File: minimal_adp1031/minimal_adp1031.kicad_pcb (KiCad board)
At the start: 4 copper layers, 39.6 x 27.9 mm, 34 parts, among them T1 ZA9644-AED, U1 ADP1031ACPZ-3-R7

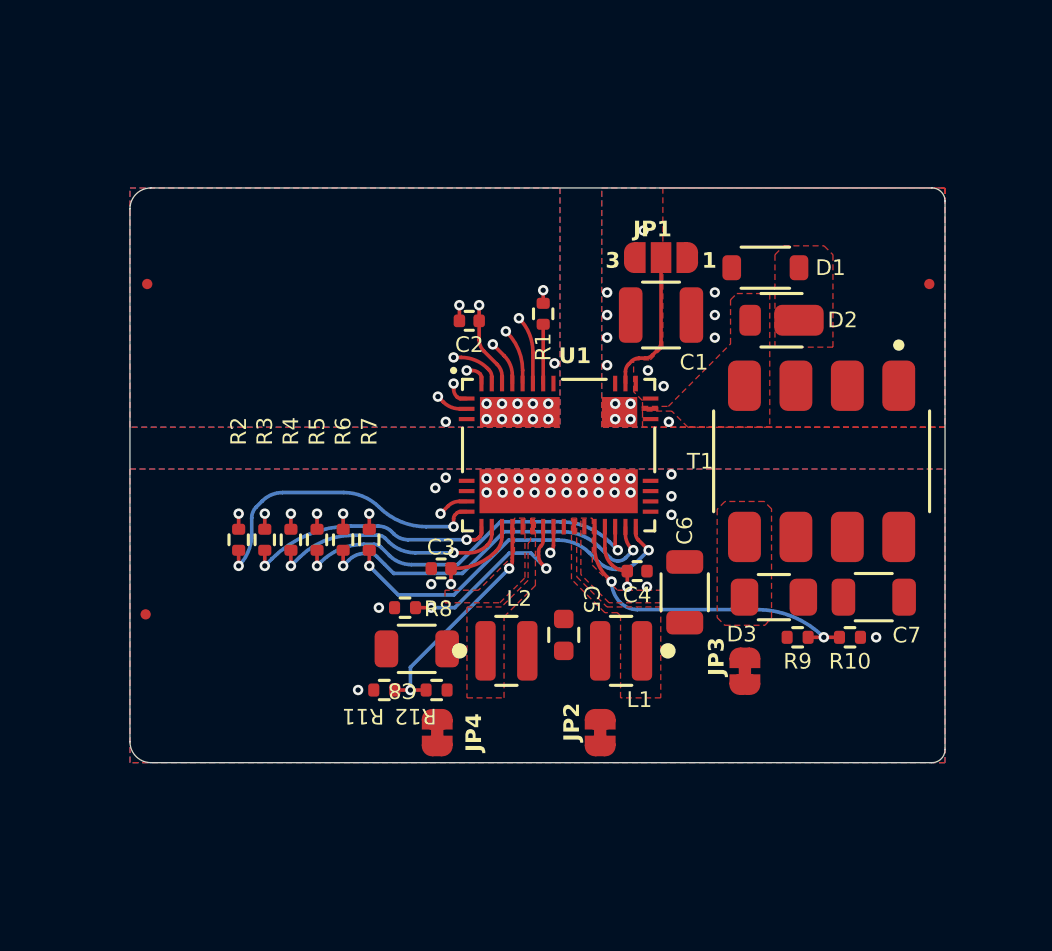
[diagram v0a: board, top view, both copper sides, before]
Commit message: backup
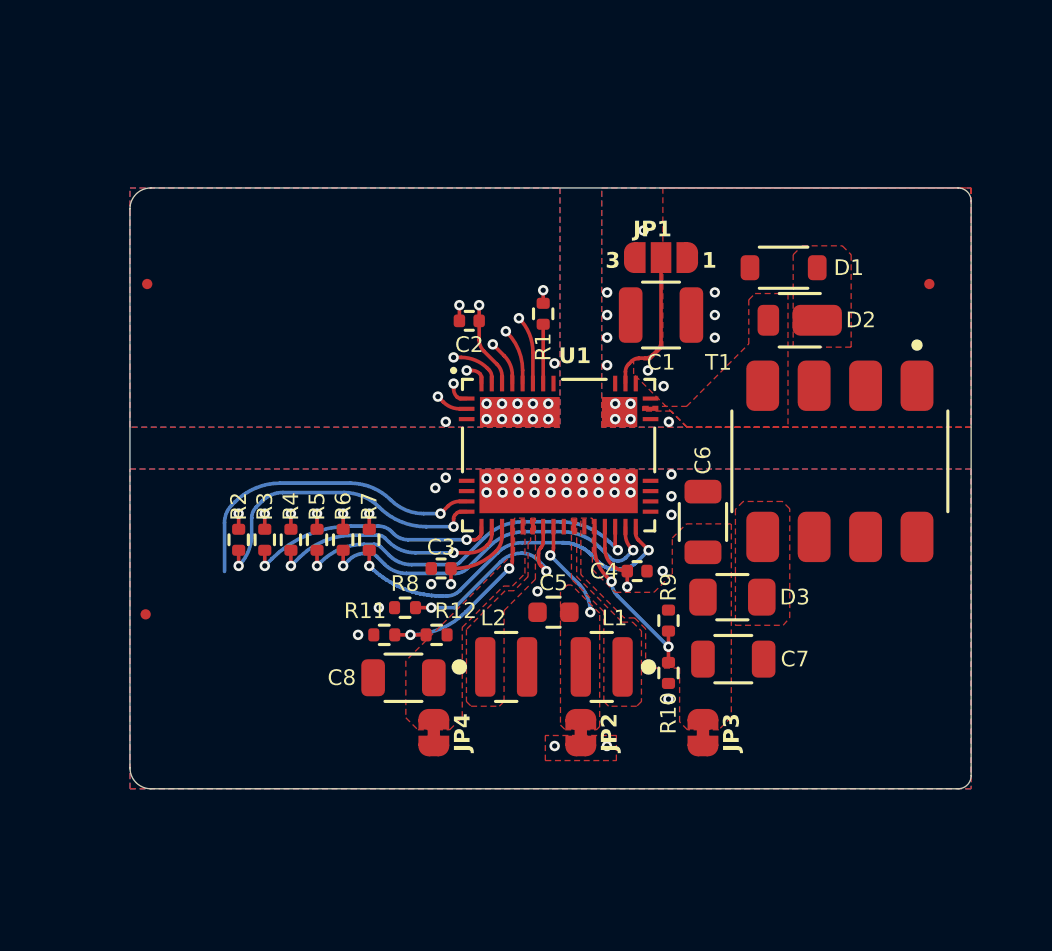
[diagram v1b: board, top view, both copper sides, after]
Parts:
- moved R10 8.99 mm to (162.1, 108.0), turned to -90 degrees
- moved C7 7.46 mm to (165.3, 107.4)
- moved R9 6.33 mm to (162.1, 105.5), turned to -90 degrees
- moved JP3 3.61 mm to (163.8, 110.9)
- moved C6 3.53 mm to (163.8, 100.7)
- moved R11 2.68 mm to (148.3, 106.2)
- moved R12 2.68 mm to (150.9, 106.2)
- moved D3 2.02 mm to (165.3, 104.3), turned to 0 degrees
- moved C8 1.55 mm to (149.3, 108.3)
- moved L1 1.23 mm to (158.9, 107.7)
- moved C5 1.21 mm to (156.6, 105.1), turned to 180 degrees
- moved JP2 0.94 mm to (157.9, 110.9)
- moved D1 0.89 mm to (167.7, 88.3)
- moved D2 0.89 mm to (168.5, 90.9)
- moved T1 0.89 mm to (170.5, 97.7)
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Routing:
- net /~{SSS}: track 1.48 -> 15.6 mm
- net /FB1: track 15.9 -> 8.70 mm
- net /VOUT2: track 1.31 -> 4.91 mm, vias 1 -> 2
- net /FB3: track 11.5 -> 9.55 mm
- net GNDA: vias 33 -> 34
- net /3V3: vias 5 -> 7
- added copper zone on F.Cu, net /3V3
- added copper zone on In1.Cu, net /3V3
- added copper zone on F.Cu, net /VOUT2
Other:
- board size 39.6 x 27.9 mm -> 40.9 x 29.2 mm

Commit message: backup
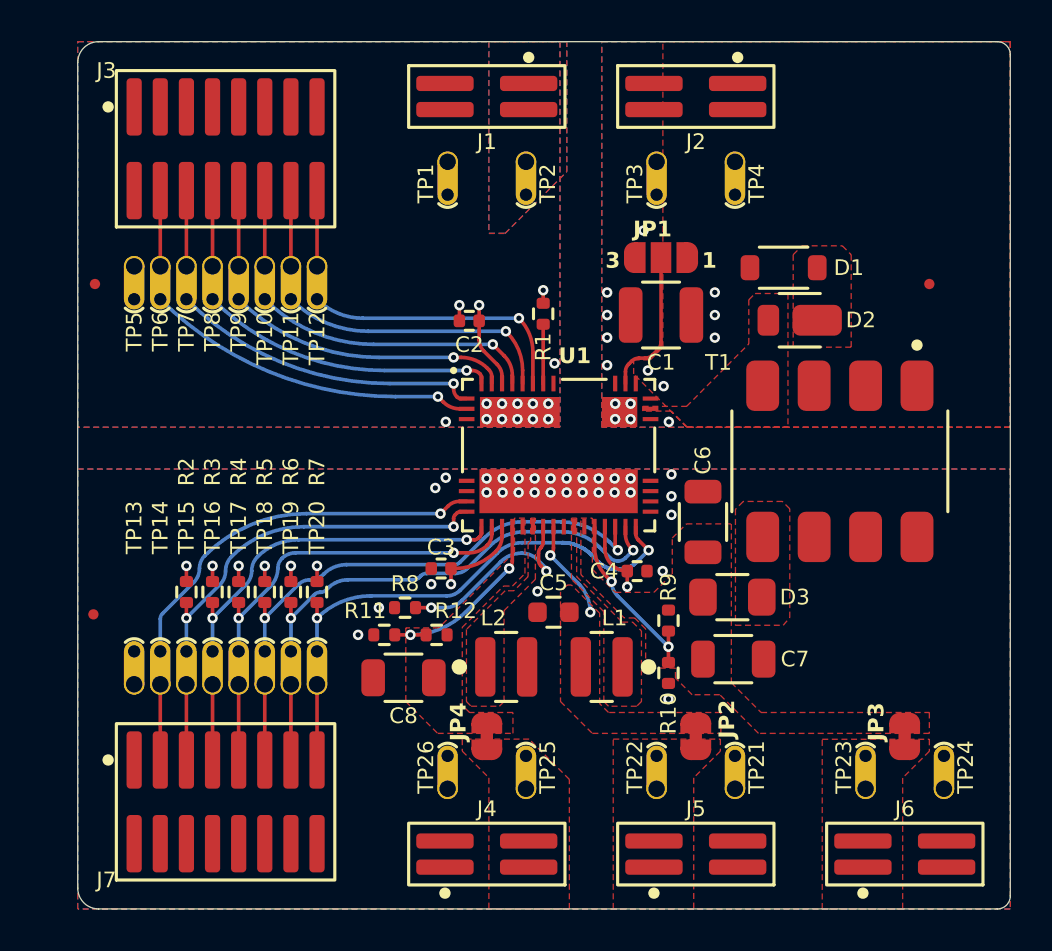
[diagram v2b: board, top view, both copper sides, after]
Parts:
- added J1: FW-02-03-G-D-085-155, connector_footprints:FW-02-03-G-D-085-155, F.Cu at (153.3, 80.0)
- added J2: FW-02-03-G-D-085-155, connector_footprints:FW-02-03-G-D-085-155, F.Cu at (163.5, 80.0)
- added J3: FW-08-03-G-D-085-155, connector_footprints:FW-08-03-G-D-085-155, F.Cu at (140.6, 82.5)
- added J4: FW-02-03-G-D-085-155, connector_footprints:FW-02-03-G-D-085-155, F.Cu at (153.3, 116.8)
- added J5: FW-02-03-G-D-085-155, connector_footprints:FW-02-03-G-D-085-155, F.Cu at (163.5, 116.8)
- added J6: FW-02-03-G-D-085-155, connector_footprints:FW-02-03-G-D-085-155, F.Cu at (173.6, 116.8)
- added J7: FW-08-03-G-D-085-155, connector_footprints:FW-08-03-G-D-085-155, F.Cu at (140.6, 114.3)
- added TP1: TestPoint, test_point_footprints:TestPoint_THTPad_Castelated, F.Cu at (151.4, 83.2)
- added TP10: TestPoint, test_point_footprints:TestPoint_THTPad_Castelated, F.Cu at (142.5, 88.3)
- added TP11: TestPoint, test_point_footprints:TestPoint_THTPad_Castelated, F.Cu at (143.8, 88.3)
- added TP12: TestPoint, test_point_footprints:TestPoint_THTPad_Castelated, F.Cu at (145.1, 88.3)
- added TP13: TestPoint, test_point_footprints:TestPoint_THTPad_Castelated, F.Cu at (136.2, 108.6)
- added TP14: TestPoint, test_point_footprints:TestPoint_THTPad_Castelated, F.Cu at (137.4, 108.6)
- added TP15: TestPoint, test_point_footprints:TestPoint_THTPad_Castelated, F.Cu at (138.7, 108.6)
- added TP16: TestPoint, test_point_footprints:TestPoint_THTPad_Castelated, F.Cu at (140.0, 108.6)
- added TP17: TestPoint, test_point_footprints:TestPoint_THTPad_Castelated, F.Cu at (141.3, 108.6)
- added TP18: TestPoint, test_point_footprints:TestPoint_THTPad_Castelated, F.Cu at (142.5, 108.6)
- added TP19: TestPoint, test_point_footprints:TestPoint_THTPad_Castelated, F.Cu at (143.8, 108.6)
- added TP2: TestPoint, test_point_footprints:TestPoint_THTPad_Castelated, F.Cu at (155.2, 83.2)
- added TP20: TestPoint, test_point_footprints:TestPoint_THTPad_Castelated, F.Cu at (145.1, 108.6)
- added TP21: TestPoint, test_point_footprints:TestPoint_THTPad_Castelated, F.Cu at (165.4, 113.7)
- added TP22: TestPoint, test_point_footprints:TestPoint_THTPad_Castelated, F.Cu at (161.6, 113.7)
- added TP23: TestPoint, test_point_footprints:TestPoint_THTPad_Castelated, F.Cu at (171.7, 113.7)
- added TP24: TestPoint, test_point_footprints:TestPoint_THTPad_Castelated, F.Cu at (175.5, 113.7)
- added TP25: TestPoint, test_point_footprints:TestPoint_THTPad_Castelated, F.Cu at (155.2, 113.7)
- added TP26: TestPoint, test_point_footprints:TestPoint_THTPad_Castelated, F.Cu at (151.4, 113.7)
- added TP3: TestPoint, test_point_footprints:TestPoint_THTPad_Castelated, F.Cu at (161.6, 83.2)
- added TP4: TestPoint, test_point_footprints:TestPoint_THTPad_Castelated, F.Cu at (165.4, 83.2)
- added TP5: TestPoint, test_point_footprints:TestPoint_THTPad_Castelated, F.Cu at (136.2, 88.3)
- added TP6: TestPoint, test_point_footprints:TestPoint_THTPad_Castelated, F.Cu at (137.4, 88.3)
- added TP7: TestPoint, test_point_footprints:TestPoint_THTPad_Castelated, F.Cu at (138.7, 88.3)
- added TP8: TestPoint, test_point_footprints:TestPoint_THTPad_Castelated, F.Cu at (140.0, 88.3)
- added TP9: TestPoint, test_point_footprints:TestPoint_THTPad_Castelated, F.Cu at (141.3, 88.3)
- moved JP3 9.81 mm to (173.6, 111.1)
- moved JP2 5.59 mm to (163.5, 111.1)
- moved R4 3.59 mm to (141.3, 104.1)
- moved R2 3.59 mm to (138.7, 104.1)
- moved R3 3.59 mm to (140.0, 104.1)
- moved R5 3.59 mm to (142.5, 104.1)
- moved R6 3.59 mm to (143.8, 104.1)
- moved R7 3.59 mm to (145.1, 104.1)
- moved JP4 2.58 mm to (153.3, 111.1)
- moved FID1 2.54 mm to (134.3, 89.1)
- moved FID2 2.54 mm to (134.2, 105.2)
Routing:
- net /~{MSS}: track 1.59 -> 20.0 mm
- net /MI: track 1.18 -> 18.9 mm
- net /MO: track 1.18 -> 18.1 mm
- net /MGPO3: track 2.23 -> 17.5 mm
- net /MCK: track 2.58 -> 17.4 mm
- net /MGPI2: track 2.75 -> 17.3 mm
- net /MGPI1: track 3.34 -> 17.1 mm
- net /SI: track 12.5 -> 21.4 mm
- net /SCK: track 12.0 -> 20.8 mm
- net /SGPI3: track 18.3 -> 26.4 mm
- net /SGPO2: track 17.9 -> 26.0 mm
- net /SGPO1: track 17.8 -> 25.5 mm
- net /~{SSS}: track 15.6 -> 22.6 mm
- net /SO: track 15.3 -> 22.2 mm
- net /3V3: vias 7 -> 5
- added copper zone on F.Cu, net /-15V0
- added copper zone on B.Cu, net /MVDD
- added copper zone on F.Cu, net /MVDD
- added copper zone on In2.Cu, net /MVDD
- added copper zone on F.Cu, net /VDD_24V
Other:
- board size 40.9 x 29.2 mm -> 45.3 x 42.2 mm

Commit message: backup
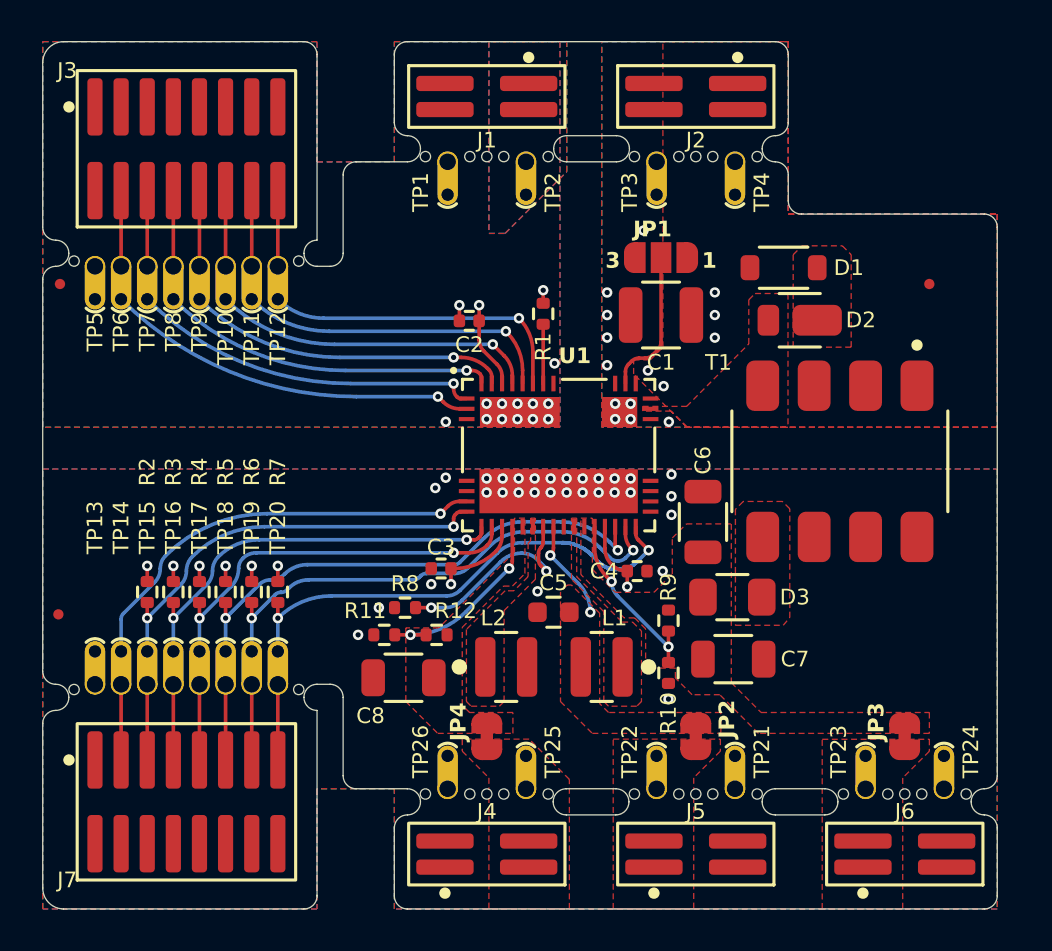
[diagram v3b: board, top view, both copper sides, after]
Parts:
- added MB1: mouse-bite-midle-50mil-200mil, mouse_bite_footprints:mouse-bite-50mil-305mil, F.Cu at (163.5, 114.3)
- added MB2: mouse-bite-midle-50mil-200mil, mouse_bite_footprints:mouse-bite-50mil-305mil, F.Cu at (173.6, 114.3)
- added MB3: mouse-bite-midle-50mil-200mil, mouse_bite_footprints:mouse-bite-50mil-305mil, F.Cu at (153.3, 114.3)
- added MB4: mouse-bite-midle-50mil-200mil, mouse_bite_footprints:mouse-bite-50mil-305mil, F.Cu at (163.5, 82.5)
- added MB5: mouse-bite-midle-50mil-200mil, mouse_bite_footprints:mouse-bite-50mil-305mil, F.Cu at (153.3, 82.5)
- added MB6: mouse-bite-50mil-450mil, mouse_bite_footprints:mouse-bite-50mil-500mil, F.Cu at (138.7, 109.2)
- added MB7: mouse-bite-50mil-450mil, mouse_bite_footprints:mouse-bite-50mil-500mil, F.Cu at (138.7, 87.6)
- U1: value ADP1031ACPZ-3-R7 -> ADP1031ACPZ-2-R7
- moved J3 1.91 mm to (138.7, 82.5)
- moved J7 1.91 mm to (138.7, 114.3)
- moved R2 1.91 mm to (136.8, 104.1)
- moved R3 1.91 mm to (138.1, 104.1)
- moved R4 1.91 mm to (139.3, 104.1)
- moved R5 1.91 mm to (140.6, 104.1)
- moved R6 1.91 mm to (141.9, 104.1)
- moved R7 1.91 mm to (143.2, 104.1)
- moved TP10 1.91 mm to (140.6, 88.3)
- moved TP11 1.91 mm to (141.9, 88.3)
- moved TP12 1.91 mm to (143.2, 88.3)
- moved TP13 1.91 mm to (134.3, 108.6)
- moved TP14 1.91 mm to (135.5, 108.6)
- moved TP15 1.91 mm to (136.8, 108.6)
- moved TP16 1.91 mm to (138.1, 108.6)
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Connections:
- net /3V3 renamed /5V0
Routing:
- net /~{SSS}: track 22.6 -> 24.5 mm
- net /~{MSS}: track 20.0 -> 21.9 mm
- net /SO: track 22.2 -> 24.1 mm
- net /SI: track 21.4 -> 23.3 mm
- net /SGPI3: track 26.4 -> 28.3 mm
- net /SCK: track 20.8 -> 22.7 mm
- net /MO: track 18.1 -> 20.0 mm
- net /MI: track 18.9 -> 20.8 mm
- net /MGPO3: track 17.5 -> 19.5 mm
- net /MGPI1: track 17.1 -> 19.0 mm
- net /MCK: track 17.4 -> 19.3 mm
- net /SGPO2: track 26.0 -> 27.9 mm
- net /MGPI2: track 17.3 -> 19.2 mm
- net /SGPO1: track 25.5 -> 27.4 mm
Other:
- board size 45.3 x 42.2 mm -> 46.4 x 42.2 mm
